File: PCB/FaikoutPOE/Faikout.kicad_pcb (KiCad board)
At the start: 2 copper layers, 42 x 69 mm, 83 parts, among them J1 RJ45_LED, J3 S21, J5 Reset, J7 TC2030-USB-NL-DS, M1 Ag9912-LP, P1 Square, Q1 BSS138PS, Q2 BSS138PS, U1 KSZ8851SNL, U2 ESP32-S3-MINI-1, U3 TCMT1100, U4 TPS62933, U5 TCMT1100, Y1 Crystal_GND24

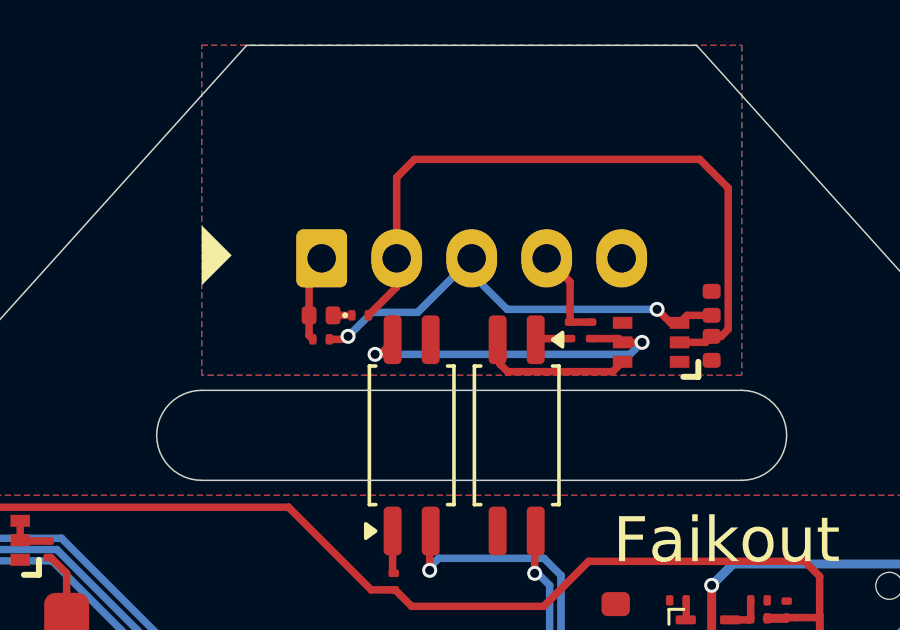
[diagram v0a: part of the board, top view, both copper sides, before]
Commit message: Tweak
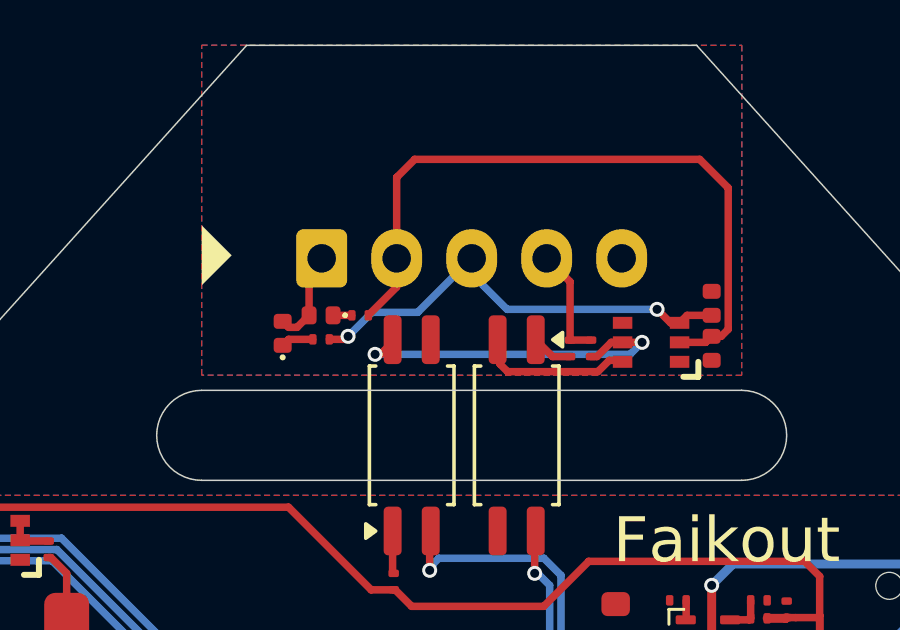
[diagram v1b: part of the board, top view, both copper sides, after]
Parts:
- added D10: D, RevK:D_0402, F.Cu at (114.7, 40.6)
- moved R10 0.60 mm to (124.3, 41.1)
- moved R6 0.60 mm to (125.0, 41.1)
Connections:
- D5 pad 2: Net-(D5-A) -> Net-(D10-A)
- J3 pad 1: Net-(D5-A) -> Net-(D10-A)
- R13 pad 1: Net-(D5-A) -> Net-(D10-K)
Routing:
- net Net-(D10-A): track 0.00 -> 3.20 mm
- net Net-(D5-A): track 2.93 -> 0.00 mm
- net Net-(D10-K): track 0.00 -> 1.09 mm
- net S21DC: track 3.15 -> 3.75 mm
